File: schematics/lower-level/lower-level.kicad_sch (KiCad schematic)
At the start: 17 parts, among them M1 Left EDF, M2 Right EDF, M3 AoA Servo MG996R, U1 STM32H743VGTx, U2 XGZP6847A, U3 XGZP6847A, U4 4525DO-DS5AI001DP, U5 ICM-42688-P, U6 MPXV7002DP, U7 MPXV7002DP, U8 BME280

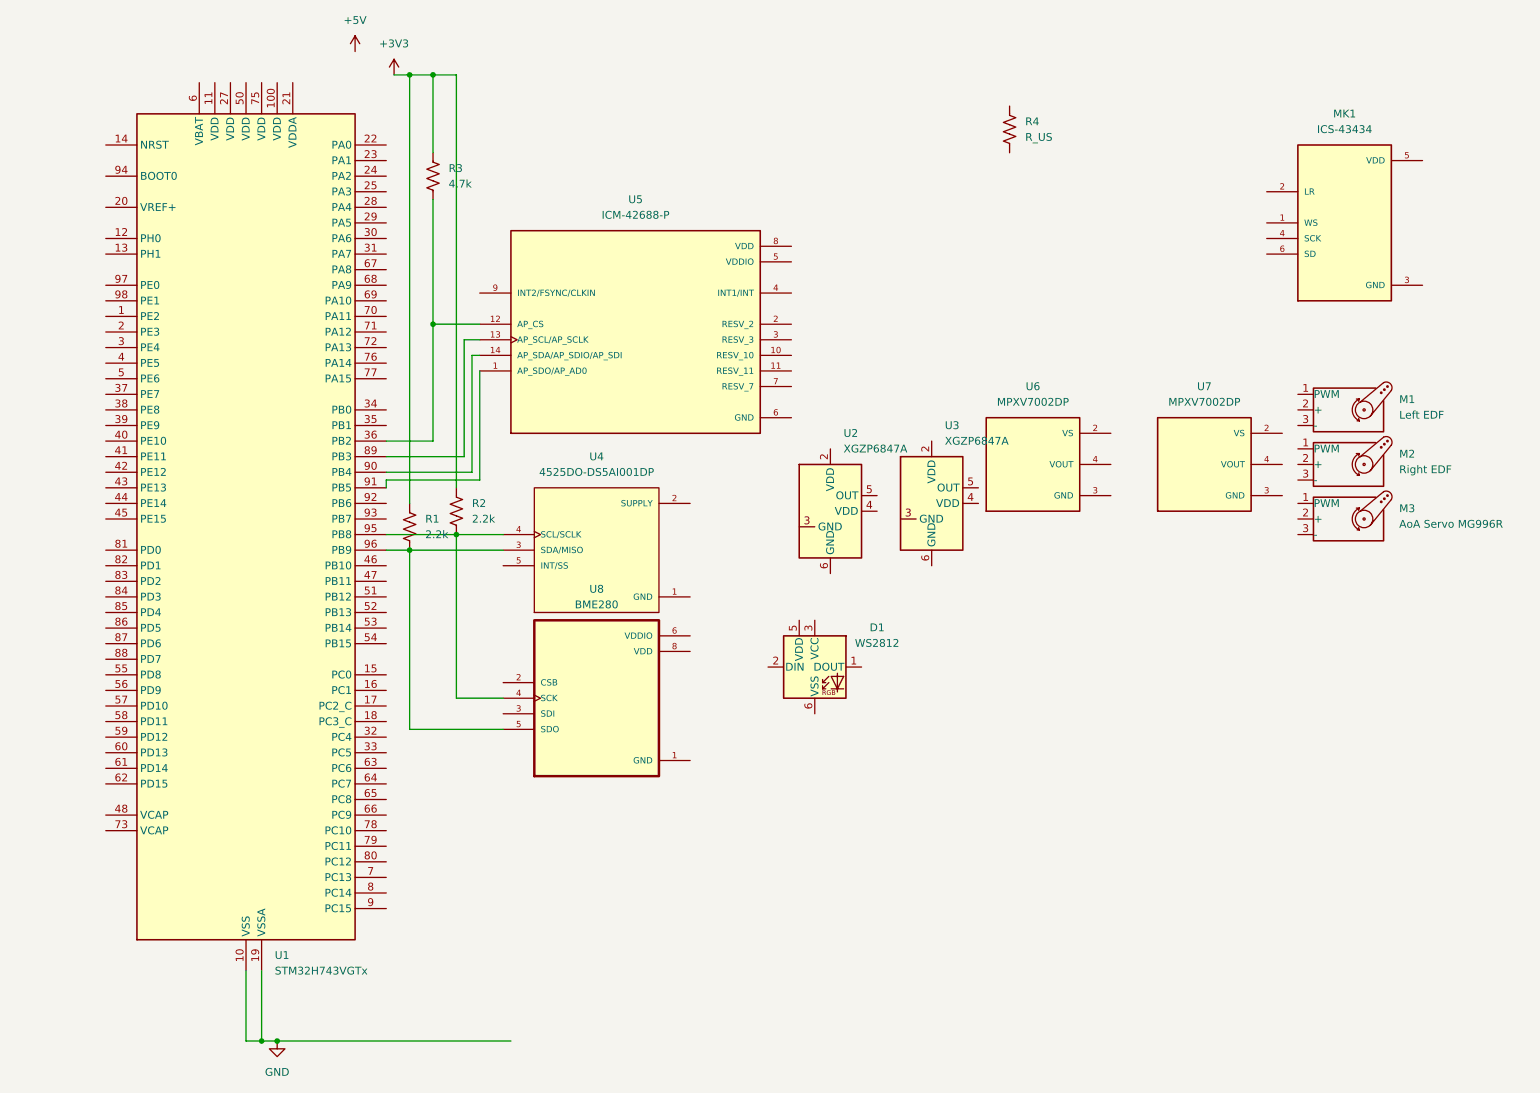
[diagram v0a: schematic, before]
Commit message: feat: schematics and basic driver code
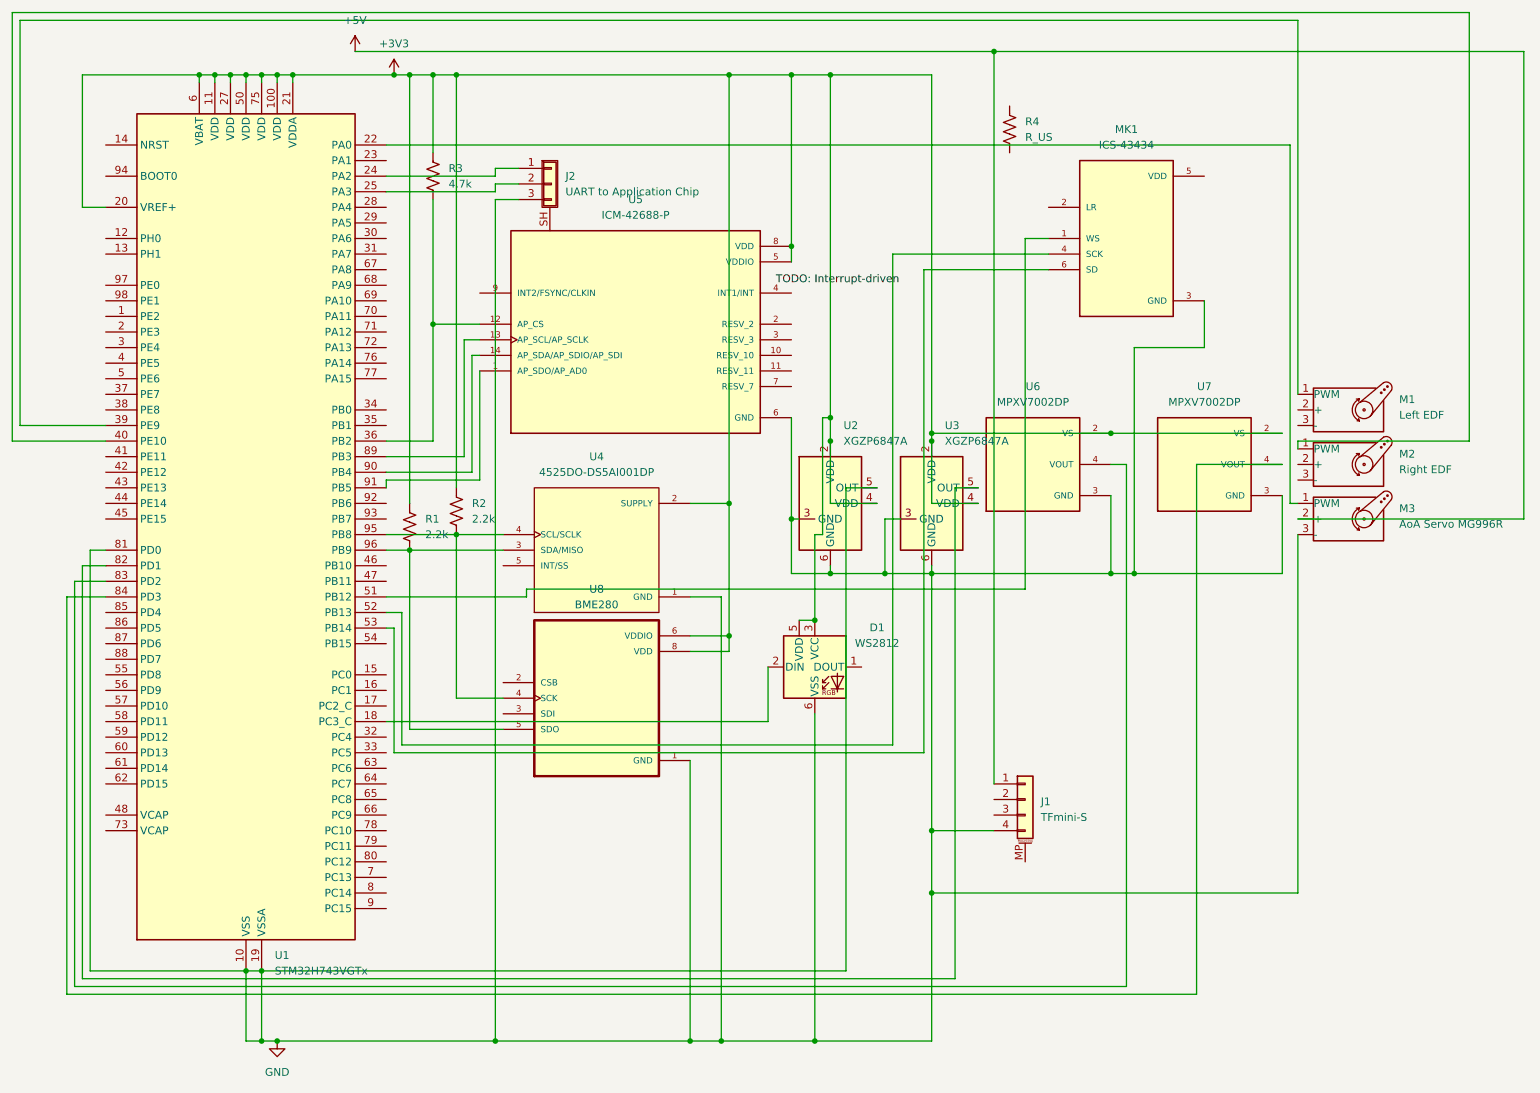
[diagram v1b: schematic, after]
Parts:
- added J1: TFmini-S, symbol Connector_Generic_MountingPin:Benewake TFmini-S
- added J2: UART to Application Chip, symbol Connector_Generic_Shielded:Conn_01x03_Shielded
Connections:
- net +3V3: now also D1.3 (VCC), D1.5 (VDD), U1.100 (VDD), U1.11 (VDD), U1.20 (VREF+), U1.21 (VDDA), U1.27 (VDD), U1.50 (VDD), U1.6 (VBAT), U1.75 (VDD), U2.2 (VDD), U2.4 (VDD), U3.2 (VDD), U3.4 (VDD), U4.2 (SUPPLY), U5.5 (VDDIO), U5.8 (VDD), U6.2 (VS), U7.2 (VS), U8.6 (VDDIO), U8.8 (VDD)
- net +5V: now also M3.2 (+), J1.1 (5V)
- net GND: now also D1.6 (VSS), M3.3 (-), MK1.3 (GND), U1.81 (PD0), U2.3 (GND), U2.5 (OUT), U2.6 (GND), U3.3 (GND), U3.6 (GND), U4.1 (GND), U5.6 (GND), U6.3 (GND), U7.3 (GND), J1.4 (GND), J2.3 (Pin_3)
- net at M3.1 (PWM): now also U1.22 (PA0)
- net at U1.18 (PC3_C): now also D1.2 (DIN)
- net at U1.24 (PA2): now also J2.1 (Pin_1)
- net at U1.25 (PA3): now also J2.2 (Pin_2)
- net at U1.39 (PE9): now also M1.1 (PWM)
- net at U1.40 (PE10): now also M2.1 (PWM)
- net at U1.51 (PB12): now also MK1.1 (WS)
- net at U1.52 (PB13): now also MK1.4 (SCK)
- net at U1.53 (PB14): now also MK1.6 (SD)
- net at U1.82 (PD1): now also U3.5 (OUT)
- net at U1.83 (PD2): now also U6.4 (VOUT)
- net at U1.84 (PD3): now also U7.4 (VOUT)
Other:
- moved on the sheet: MK1, U2
